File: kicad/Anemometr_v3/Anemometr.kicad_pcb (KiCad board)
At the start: 2 copper layers, 45 x 45 mm, 170 parts, among them J1 TxD, J10 +Z1, J11 +Z2, J12 +Z3, J13 +Z4, J14 -Z1, J15 -Z2, J16 -Z3, J17 -Z4, J18 1 TxD+, J19 2 TxD-, J2 RxD, J20 3 RxD+, J21 4-5, J22 6 RxD-, J23 7-8, J24 Conn_01x01_Female, J25 Conn_01x01_Female, J26 Conn_01x01_Female, J3 SCL, J4 SDA, J5 RST, J6 +EXT, J7 -EXT, J8 SWD, J9 SWC, Q1 5N10, U1 STM32F103C8Tx, U2 TS5A3166DBVR, U3 TS5A3166DBVR, U4 LMR14206, U5 TS5A3166DBVR, U6 NCP1117-3.3, U7 TS5A3166DBVR, U8 MCP1703-3.3, U9 MCP1703-3.3, Y1 CSTCE8M00G52A-R0, Y2 ECS-250-20-33

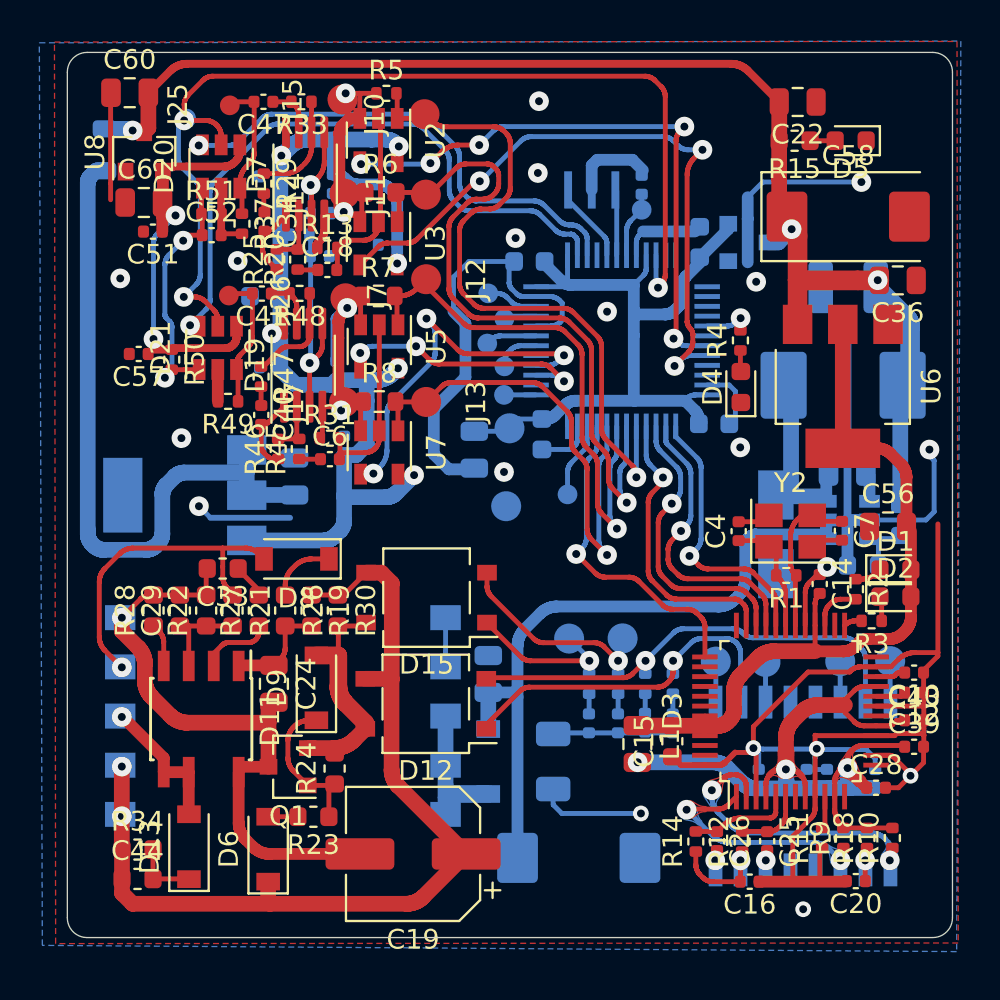
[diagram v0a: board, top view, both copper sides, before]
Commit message: изменено:      kicad/Anemometr_v3/Anemometr.kicad_pcb 	изменено:      kicad/Anemometr_v3/Anemometr.kicad_pcb-bak
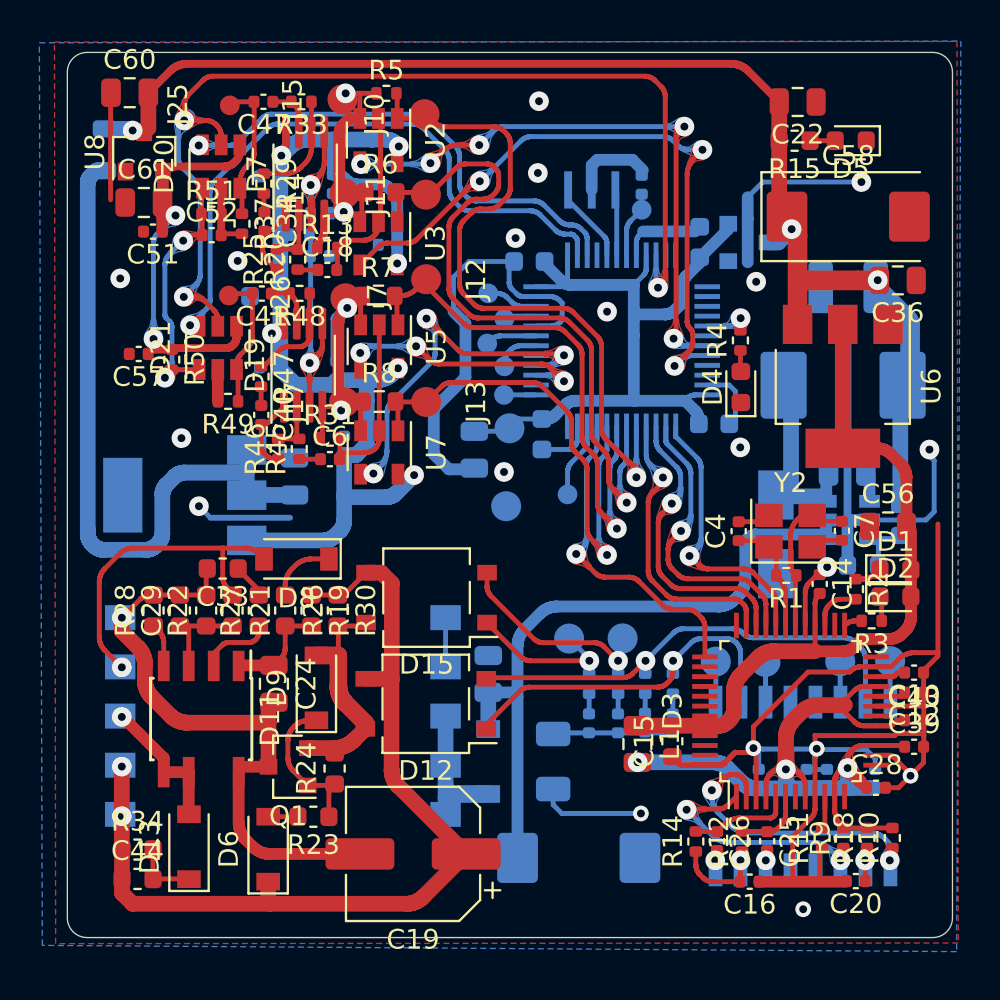
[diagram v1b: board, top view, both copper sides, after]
